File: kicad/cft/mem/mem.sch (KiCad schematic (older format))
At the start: 9 parts

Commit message: Planning and design for the MEM board.
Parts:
- added U104: 74HC138, alexios:SOIC-16, symbol alexios:74HC138
- added U111, U112: 29W040, Sockets:PLCC32, symbol Memory_Flash:29W040
- U101, U102, U105, U106, U107, U108, U109, U110: renamed from U?; footprint Package_SO:SOJ-36_10.16x23.49mm_P1.27mm -> Package_DIP:DIP-40_W15.24mm
- U103: renamed from U?; footprint (none) -> alexios:SOIC-16
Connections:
- net labels added: AB19, AB20, AB21, AB22, AB23, DB10, DB11, DB12, DB13, DB14, DB15, DB8, DB9, ~RBCE4, ~RBCE5, ~RBCE6, ~RBCE7, ~ROMCE
- net labels removed: PB10, PB11, PB12, PB13, PB14, PB15, PB8, PB9
- wire segments 300 -> 373
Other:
- note added: "Notes"
- note added: "Use DIP40 sockets for first 1024×16 bank of SRAM (four 512K chips), then\nleave land patterns for another 7M in smaller packages, SOJ or Flash TSSOP.\n\nThis implies only one MEM board need be used. RAM can be mapped to\n00:0000–0F:FFFF for the first (DIP) Megaword, then extending up to 7F:FFFF\nwith all 8 Megawords installed.\n\nFlash devices are in PLCC32 sockets and form a single 512K×16 ROM B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"

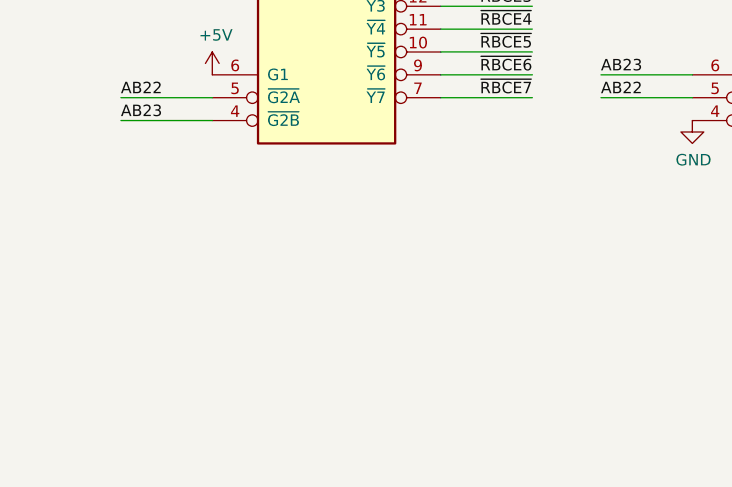
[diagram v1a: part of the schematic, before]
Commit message: Play around with new MEM board
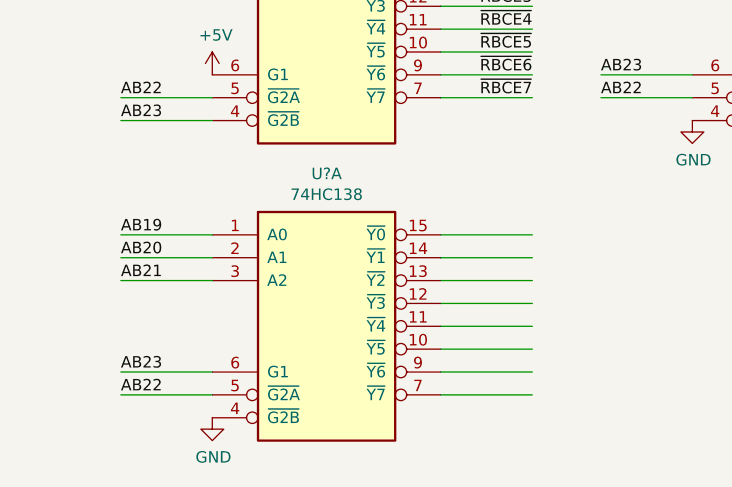
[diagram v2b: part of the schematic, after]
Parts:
- added U?: 74HC138, alexios:SOIC-16, symbol alexios:74HC138
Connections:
- wire segments 373 -> 386
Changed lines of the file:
@@
 EESchema Schematic File Version 4
 LIBS:mem-cache
-EELAYER 26 0
+EELAYER 30 0
 EELAYER END
 $Descr A3 16535 11693
@@
 Text Label 5250 7650 2    50   ~ 0
 ~ROMCE
-Wire Bus Line
-	15050 3050 15050 3350
-Wire Bus Line
-	15050 3450 15050 3750
 Text Notes 6700 8050 0    100  ~ 20
 Notes
 Text Notes 6700 8900 0    50   ~ 0
 Use DIP40 sockets for first 1024×16 bank of SRAM (four 512K chips), then\nleave land patterns for another 7M in smaller packages, SOJ or Flash TSSOP.\n\nThis implies only one MEM board need be used. RAM can be mapped to\n00:0000–0F:FFFF for the first (DIP) Megaword, then extending up to 7F:FFFF\nwith all 8 Megawords installed.\n\nFlash devices are in PLCC32 sockets and form a single 512K×16 ROM Bank\nmapped to 80:0000–87:FFFF. This is hardwired.
+Wire Wire Line
+	1750 8950 1350 8950
+Wire Wire Line
+	1750 9050 1350 9050
+Wire Wire Line
+	1750 9150 1350 9150
+Wire Wire Line
+	1750 9650 1350 9650
+Wire Wire Line
+	1750 9550 1350 9550
+Text Label 1350 9550 0    50   ~ 0
+AB23
+Wire Wire Line
+	3150 8950 2750 8950
+Wire Wire Line
+	3150 9050 2750 9050
+Wire Wire Line
+	3150 9150 2750 9150
+Wire Wire Line
+	3150 9550 2750 9550
+Wire Wire Line
+	3150 9650 2750 9650
+Wire Wire Line
+	2750 9250 3150 9250
+Wire Wire Line
+	2750 9350 3150 9350
+Wire Wire Line
+	2750 9450 3150 9450
+$Comp
+L alexios:74HC138 U?
+U 1 1 5D65AD6B
+P 2250 9350
+F 0 "U?" H 2250 10017 50  0000 C CNN
+F 1 "74HC138" H 2250 9926 50  0000 C CNN
+F 2 "alexios:SOIC-16" H 2250 9350 50  0001 C CNN
+F 3 "http://www.ti.com/lit/gpn/sn74LS138" H 2250 9350 50  0001 C CNN
+	1    2250 9350
+	1    0    0    -1
+$EndComp
+Text Label 1350 9650 0    50   ~ 0
+AB22
+Text Label 1350 9150 0    50   ~ 0
+AB21
+Text Label 1350 9050 0    50   ~ 0
+AB20
+Text Label 1350 8950 0    50   ~ 0
+AB19
+$Comp
+L power:GND #PWR?
+U 1 1 5D6FAE34
+P 1750 9750
+F 0 "#PWR?" H 1750 9500 50  0001 C CNN
+F 1 "GND" H 1755 9577 50  0000 C CNN
+F 2 "" H 1750 9750 50  0001 C CNN
+F 3 "" H 1750 9750 50  0001 C CNN
+	1    1750 9750
+	1    0    0    -1
+$EndComp
+Wire Bus Line
+	15050 3450 15050 3750
+Wire Bus Line
+	15050 3050 15050 3350
 $EndSCHEMATC

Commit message: Experimenting with MEM board configurations and layouts.
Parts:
- removed U101, U102, U105, U106, U107, U108, U109, U110: IS64C5128AL-12KLA3, Package_DIP:DIP-40_W15.24mm, symbol Memory_RAM:IS64C5128AL-12KLA3
- removed U?: 74HC138, alexios:SOIC-16, symbol alexios:74HC138
- renumbered U111 to U1, U112 to U2, U103 to U3, U104 to U4
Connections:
- net labels added: AB[0..18]
- wire segments 386 -> 169
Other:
- moved on the sheet: U1, U2, U3A, U4A

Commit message: Working on MEM board.
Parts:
- added JP101: Jumper_3_Bridged12, Connector_PinHeader_2.54mm:PinHeader_1x03_P2.54mm_Vertical, symbol Jumper:Jumper_3_Bridged12
- added U29: 74HC138, alexios:SOIC-16, symbol alexios:74HC138
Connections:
- net labels added: ~CS0, ~CS1, ~CS10, ~CS11, ~CS2, ~CS3, ~CS4, ~CS5, ~CS6, ~CS7, ~CS8, ~CS9, ~ROMCS, ~ROMWE
- net labels removed: ~RBCE0, ~RBCE1, ~RBCE2, ~RBCE3, ~RBCE4, ~RBCE5, ~RBCE6, ~RBCE7, ~ROMCE
- wire segments 169 -> 186
- no-connect marks 10 -> 14
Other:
- note added: "AB=00AAAxxx:xxxxxxxx:xxxxxxxx\n(0–4096K, chunks of 512K)"
- note added: "AB=01AAAxxx:xxxxxxxx:xxxxxxxx\n(4096–8192K, chunks of 512K)"
- moved on the sheet: U1, U2
